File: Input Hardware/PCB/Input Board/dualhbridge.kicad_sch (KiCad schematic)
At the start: 10 parts, among them U2 DRV8837, U3 DRV8837, U4 DRV8837, U5 DRV8837

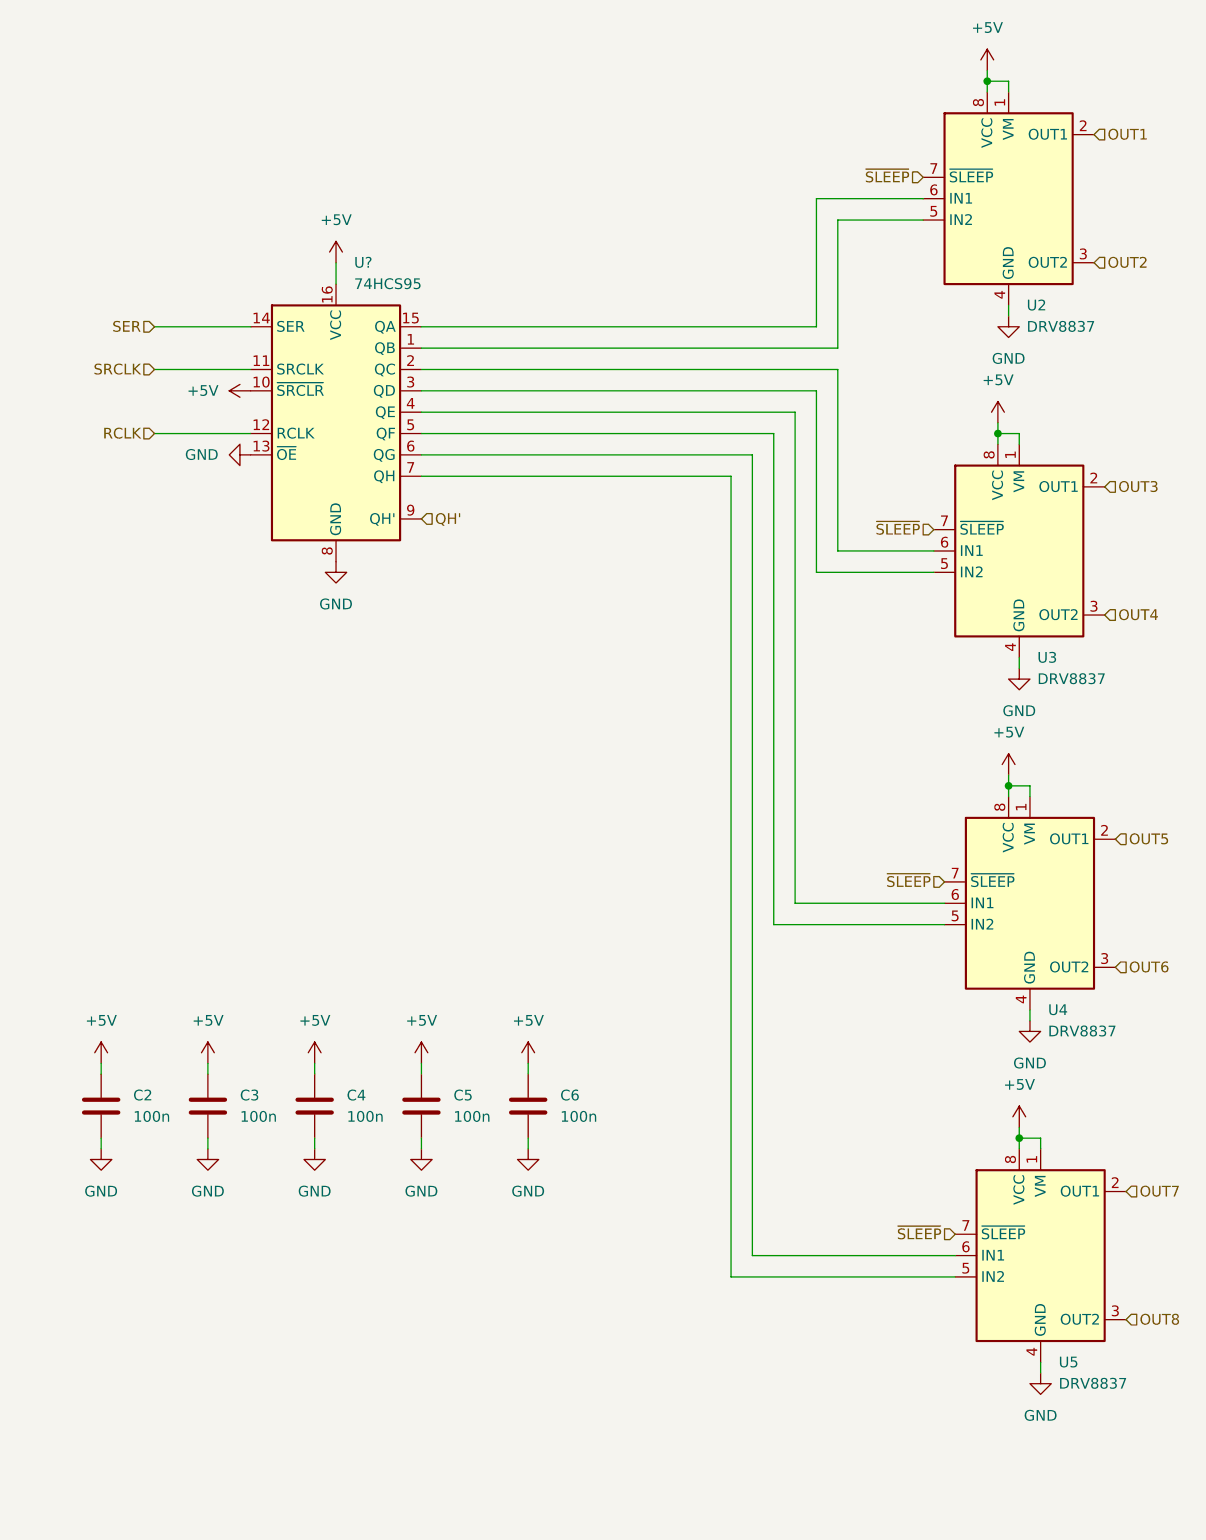
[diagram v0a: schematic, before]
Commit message: Schematic Cleanup
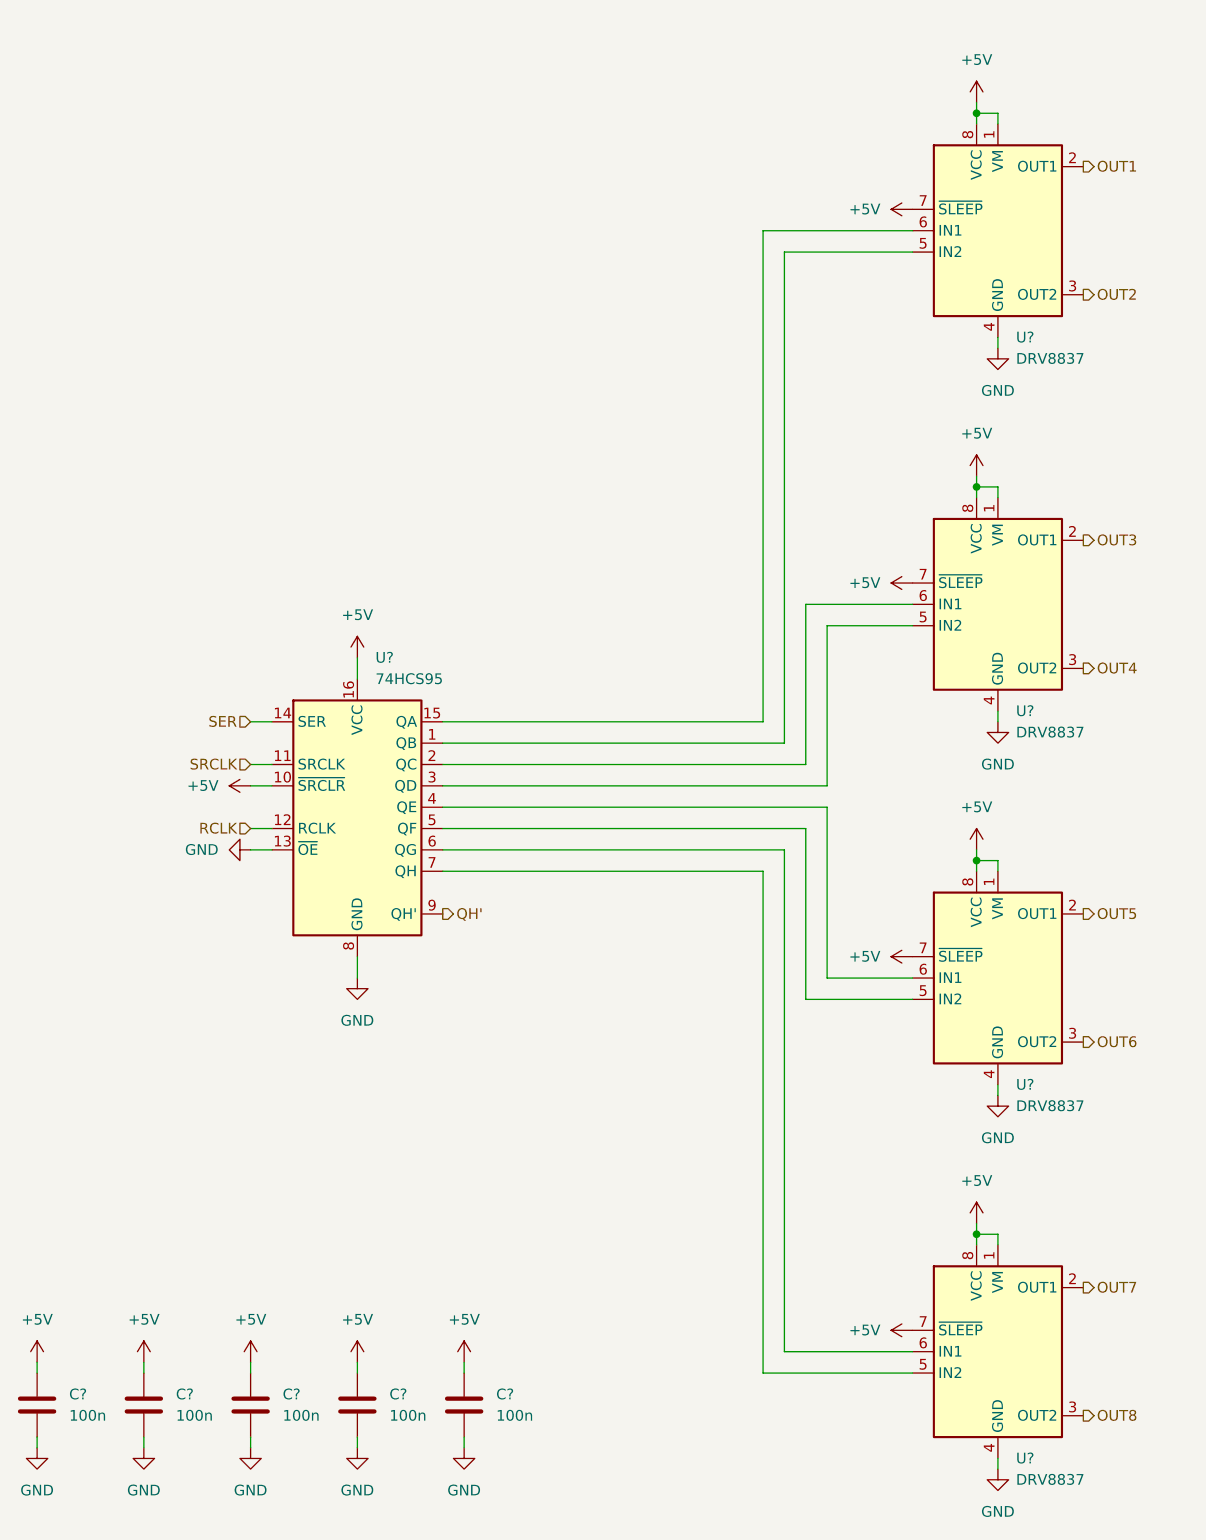
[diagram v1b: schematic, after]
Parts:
- renumbered C3 to C?, C2 to C?, C5 to C?, C4 to C?, C6 to C?, U5 to U?, U2 to U?, U4 to U?, U3 to U?
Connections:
- net ~{SLEEP} is gone; now on net +5V: U?.7 (~{SLEEP}), U?.7 (~{SLEEP}), U?.7 (~{SLEEP}), U?.7 (~{SLEEP})
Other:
- moved on the sheet: C?, U?
